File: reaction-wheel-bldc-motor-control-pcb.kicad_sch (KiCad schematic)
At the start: 50 parts, among them J1 Conn_01x04_Pin, J2 Conn_01x04_Pin, J3 Conn_01x03_Pin, J4 USB_C_Receptacle_USB2.0_16P, J5 Conn_01x04_Pin, J6 Conn_01x06_Pin, SW1 SW_SPST, U1 USBLC6-2SC6, U2 STM32G431CBUx, U3 AS5047D, U4 DRV8311H, U5 SN65HVD231, U6 TPS562200, Y1 16MHz

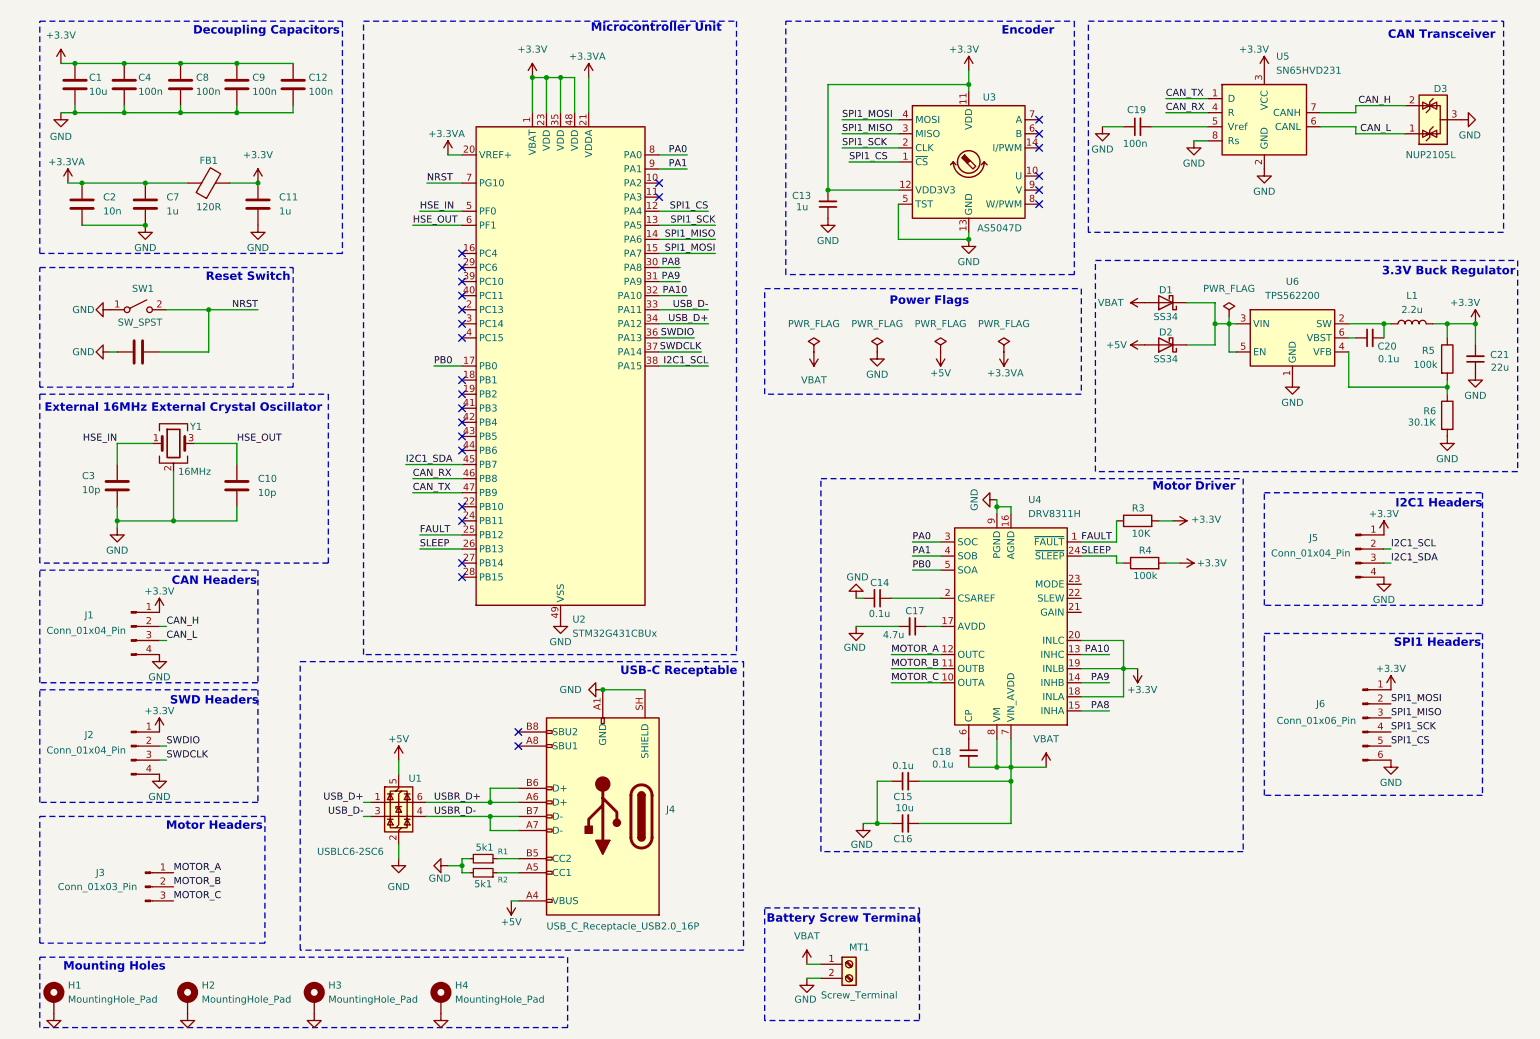
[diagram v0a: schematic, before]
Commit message: routing almost finished
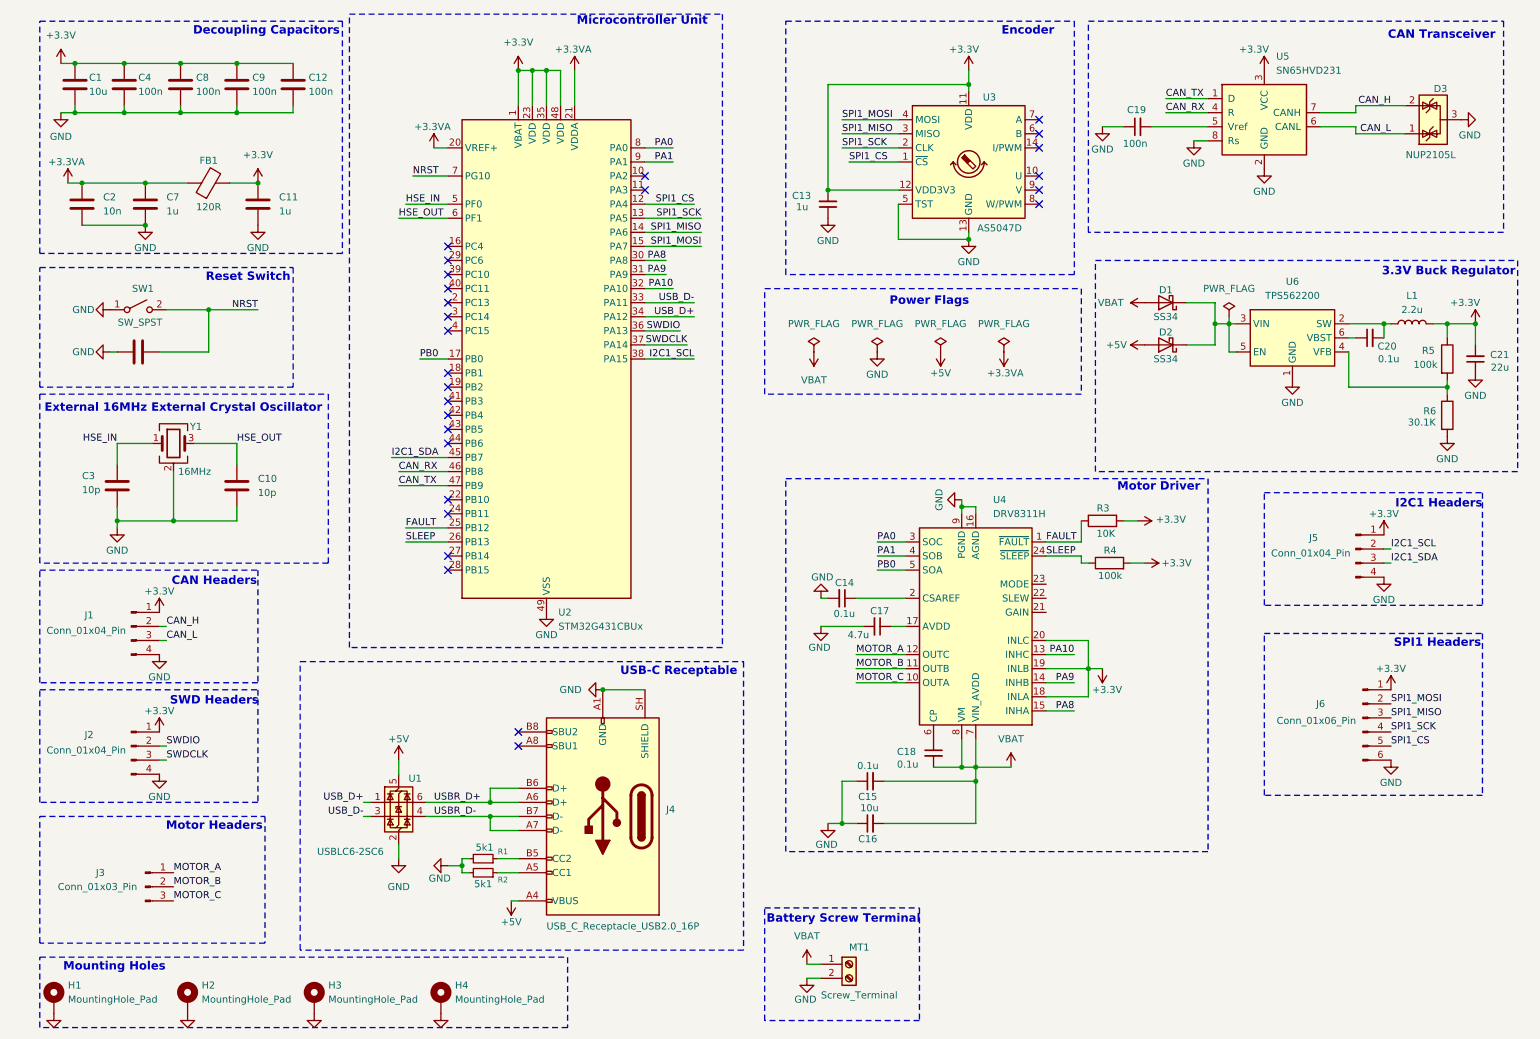
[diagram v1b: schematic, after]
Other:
- moved on the sheet: C14, C15, C16, C17, C18, R3, R4, U2, U4
